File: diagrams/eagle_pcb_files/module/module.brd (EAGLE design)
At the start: 60 x 60 mm, 3 parts

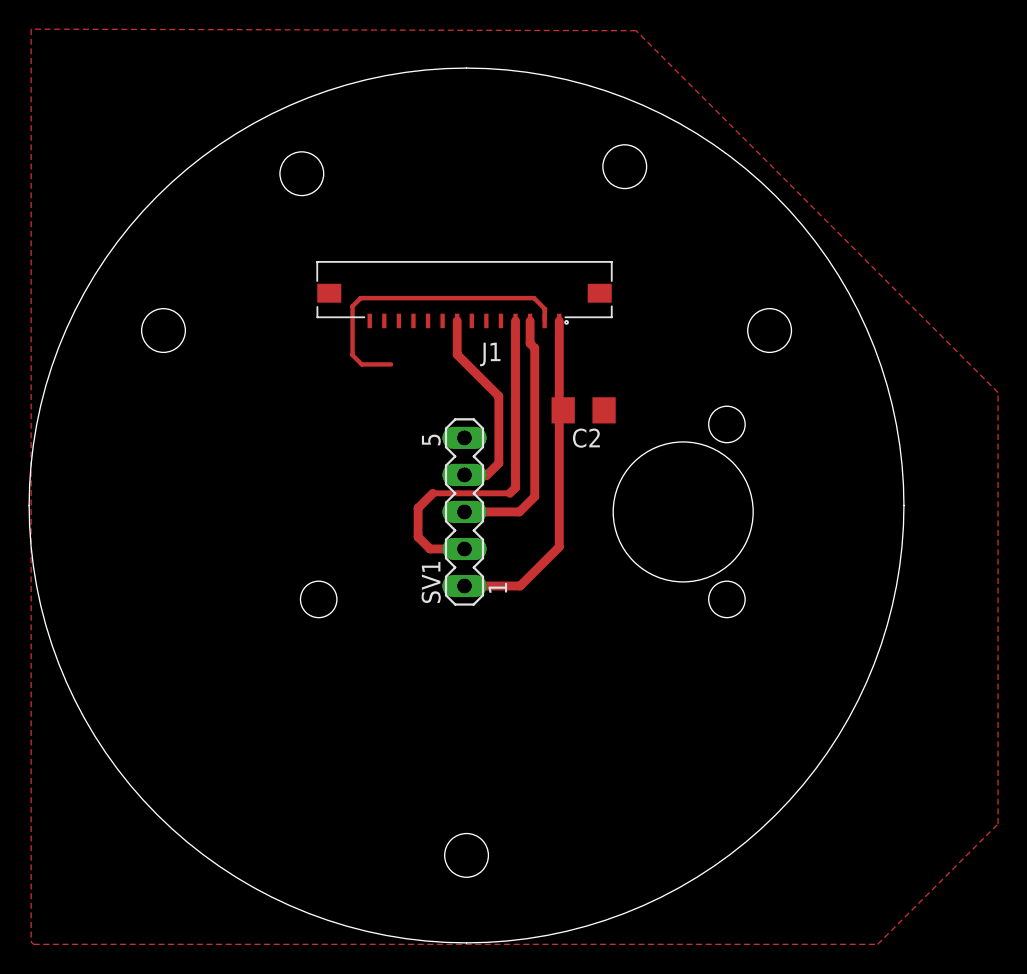
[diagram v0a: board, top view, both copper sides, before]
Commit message: Some features added
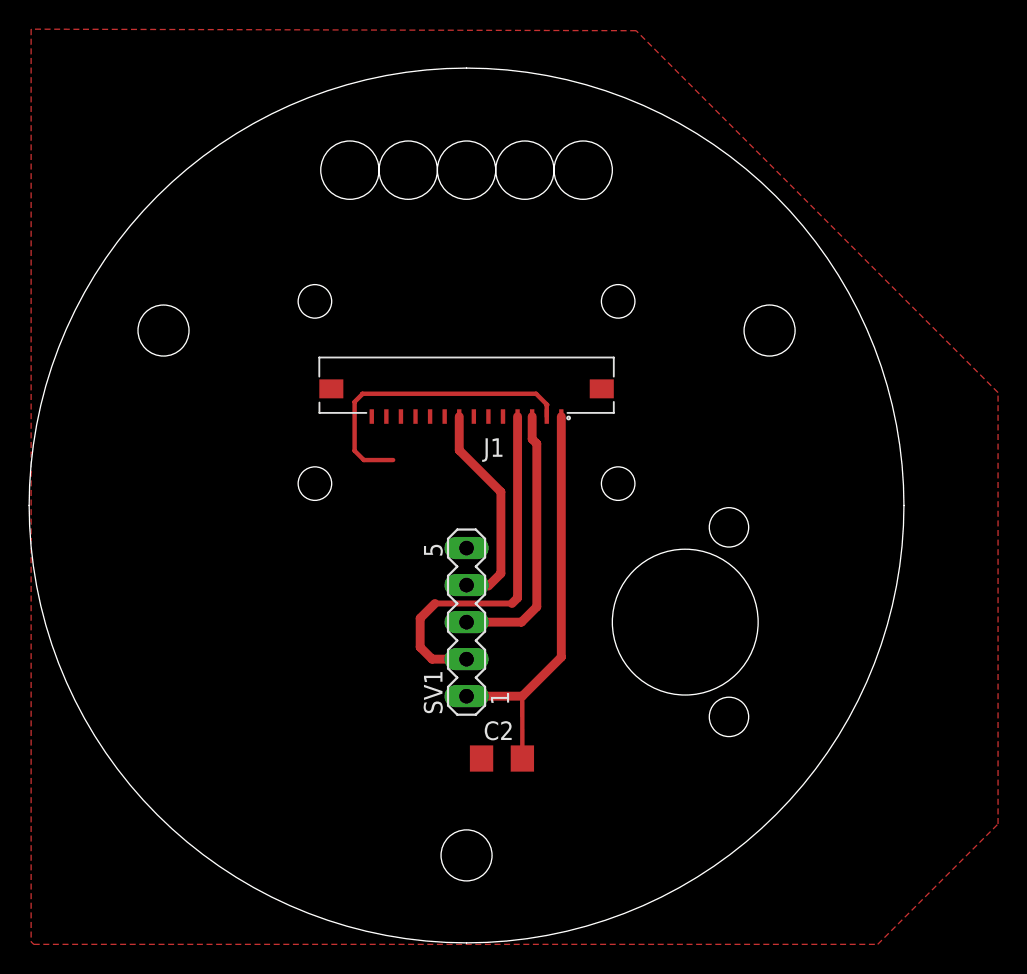
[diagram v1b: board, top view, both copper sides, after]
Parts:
- moved C2 24.5 mm to (42.4, 12.6), turned to 0 degrees
- moved SV1 7.56 mm to (40.0, 22.0)
- moved J1 6.56 mm to (40.0, 38.0)
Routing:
- net VCC: track 23.4 -> 28.4 mm
- net INT: track 13.7 -> 14.7 mm
- net SCL: track 17.4 -> 18.4 mm
- net SDA: track 24.2 -> 25.2 mm
